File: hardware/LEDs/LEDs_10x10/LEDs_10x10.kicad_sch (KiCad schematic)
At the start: 106 parts, among them J2 Conn_01x03_Pin, J3 Conn_01x02_Pin, Q2 NPN, U1 OPA735

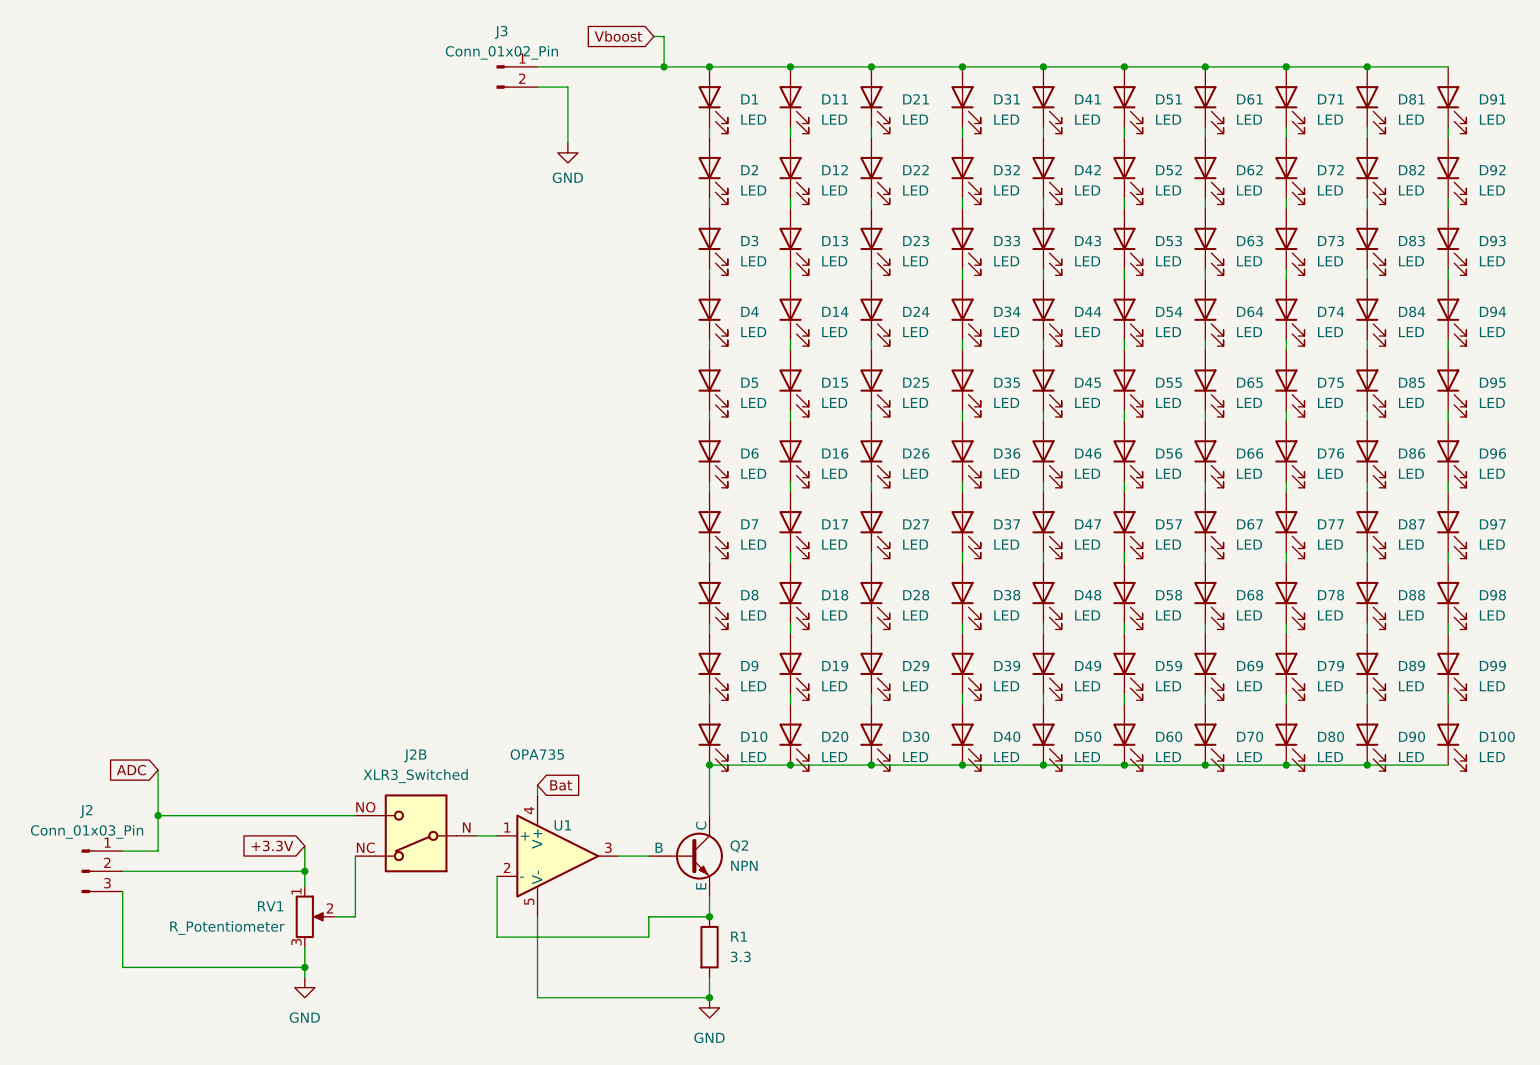
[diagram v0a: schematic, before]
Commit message: pcb
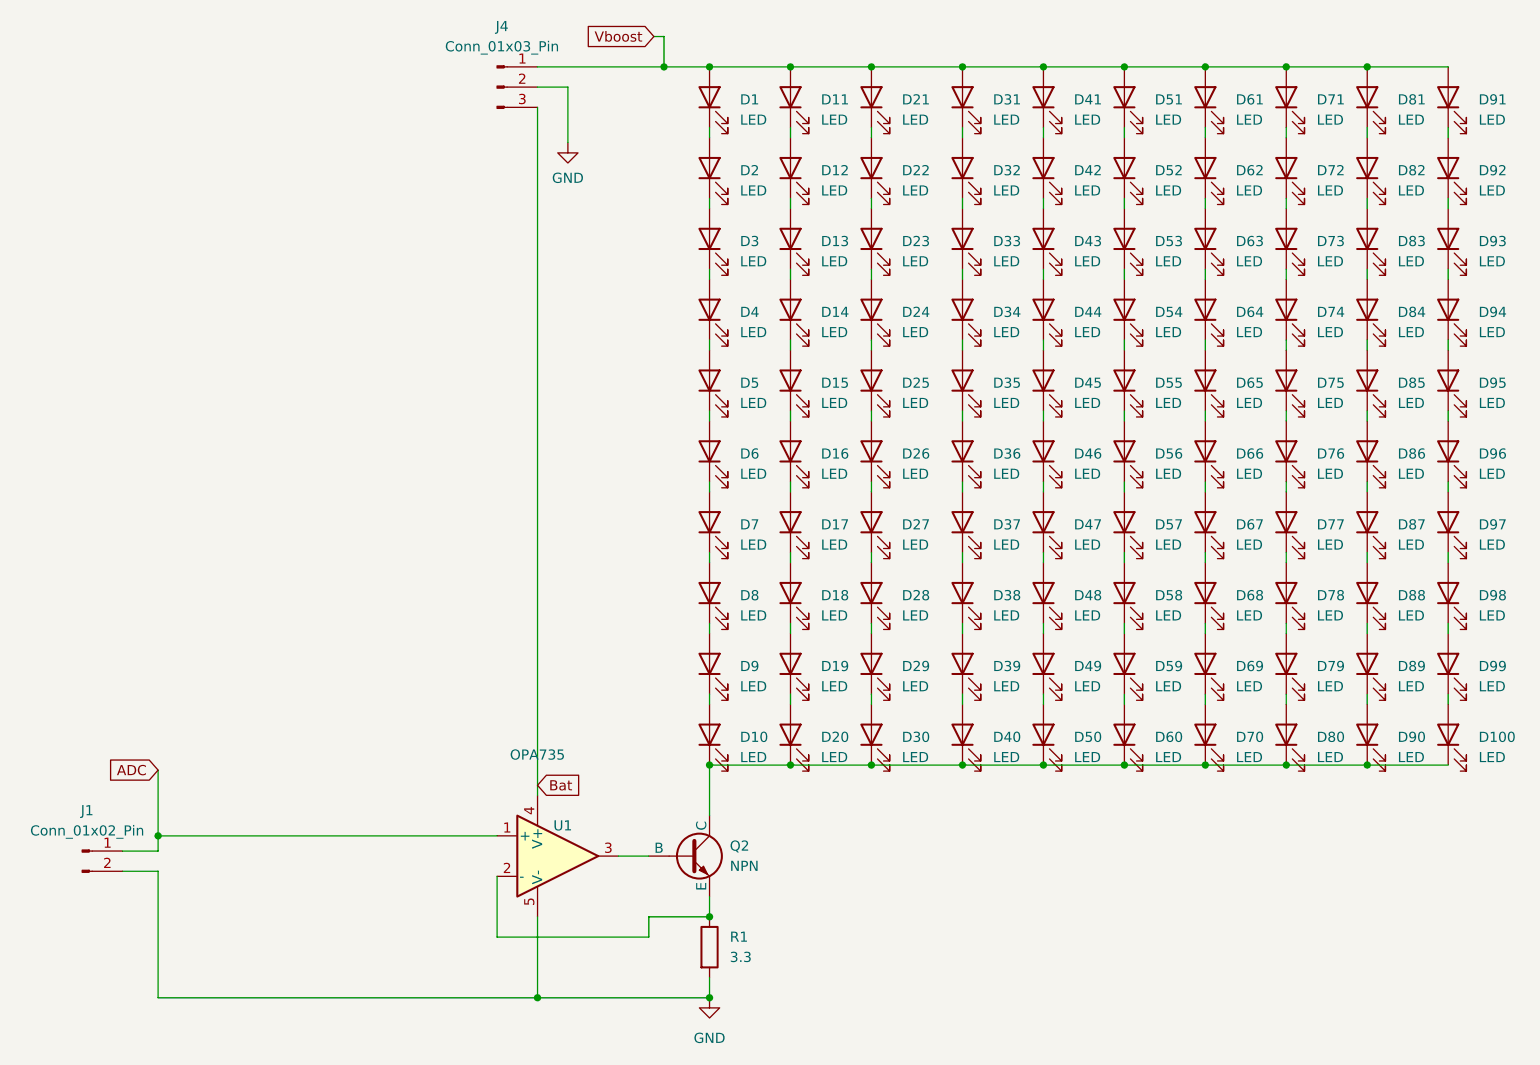
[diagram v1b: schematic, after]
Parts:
- removed J2: Conn_01x03_Pin, symbol Connector:Conn_01x03_Pin
- removed J3: Conn_01x02_Pin, symbol Connector:Conn_01x02_Pin
- removed RV1: R_Potentiometer, symbol Device:R_Potentiometer
- added J1: Conn_01x02_Pin, symbol Connector:Conn_01x02_Pin
- added J4: Conn_01x03_Pin, symbol Connector:Conn_01x03_Pin
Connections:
- net ADC: now also U1.1 (+), J1.1 (Pin_1)
- net Bat: now also J4.3 (Pin_3)
- net GND: now also J1.2 (Pin_2), J4.2 (Pin_2)
- net Vboost: now also J4.1 (Pin_1)
